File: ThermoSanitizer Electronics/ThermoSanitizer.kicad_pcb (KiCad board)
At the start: 2 copper layers, 86.4 x 59.7 mm, 17 parts, among them J1 5V_Thermo, J2 9V_In, J3 Ultrasonic, J5 Motor_Out, Q1 IRF540N, U1 L7805

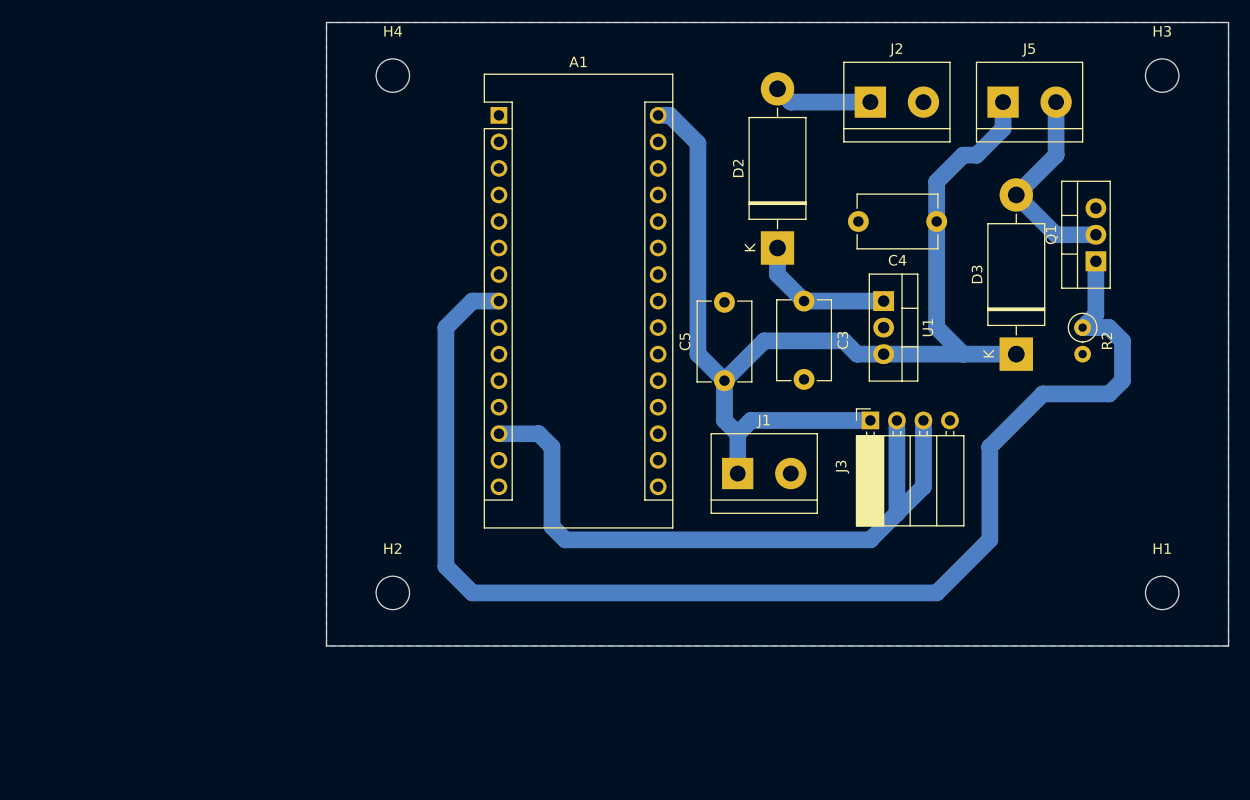
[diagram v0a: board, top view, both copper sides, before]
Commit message: Adding alot of stuff
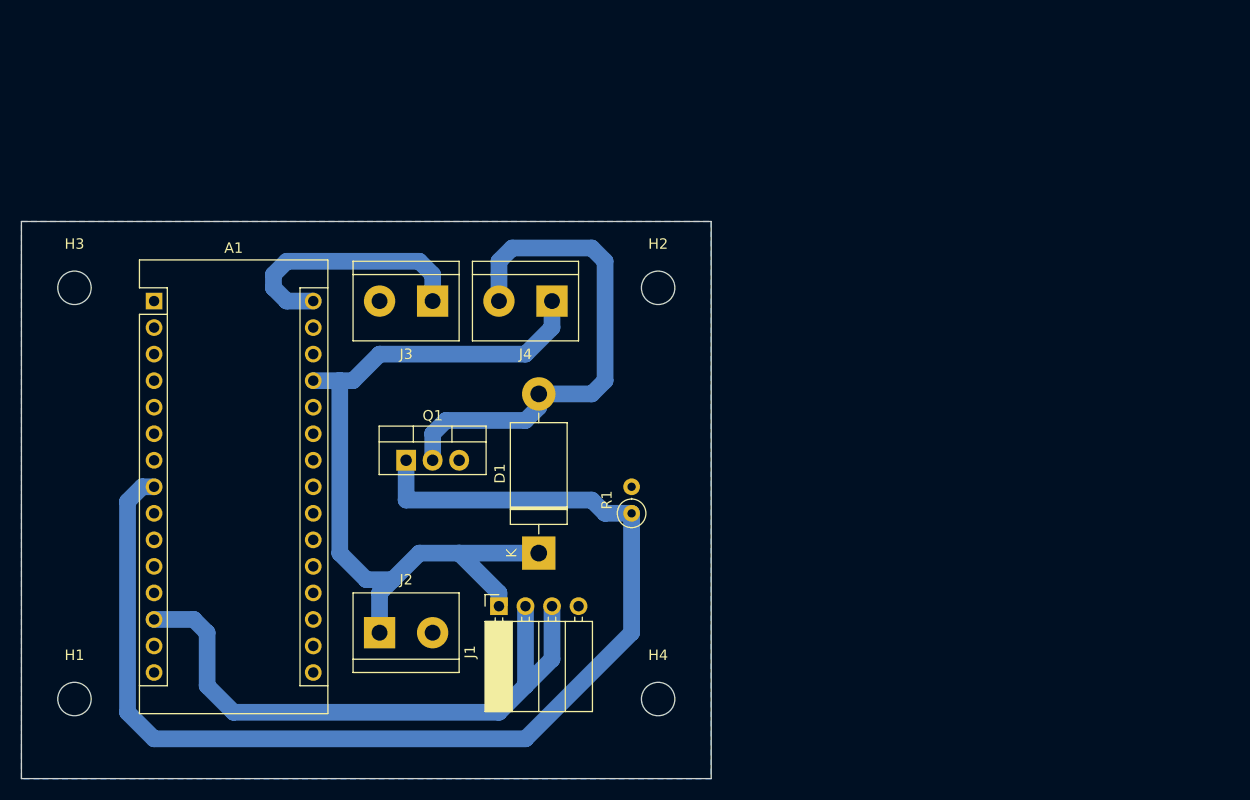
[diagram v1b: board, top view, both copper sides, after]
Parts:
- removed C3: 10uF, Capacitor_THT:C_Disc_D7.5mm_W5.0mm_P7.50mm
- removed C4: 0.1uF, Capacitor_THT:C_Disc_D7.5mm_W5.0mm_P7.50mm
- removed C5: 1uF, Capacitor_THT:C_Disc_D7.5mm_W5.0mm_P7.50mm
- removed D2, D3: 1N5400, Diode_THT:D_DO-201AD_P15.24mm_Horizontal
- removed J5: Motor_Out, TerminalBlock:TerminalBlock_bornier-2_P5.08mm
- removed R2: 1K, Resistor_THT:R_Axial_DIN0207_L6.3mm_D2.5mm_P2.54mm_Vertical
- removed U1: L7805, Package_TO_SOT_THT:TO-220-3_Vertical
- added D1: 1N5400, Diode_THT:D_DO-201AD_P15.24mm_Horizontal, F.Cu at (91.4, 97.8)
- added J4: Motor_Out, TerminalBlock:TerminalBlock_bornier-2_P5.08mm, F.Cu at (92.7, 73.7)
- added R1: 1K, Resistor_THT:R_Axial_DIN0207_L6.3mm_D2.5mm_P2.54mm_Vertical, F.Cu at (100.3, 94.0)
- H1, H2, H3, H4: value MountingHole_Pad -> MountingHole
- J1: value 5V_Thermo -> Ultrasonic; footprint TerminalBlock:TerminalBlock_bornier-2_P5.08mm -> Connector_PinSocket_2.54mm:PinSocket_1x04_P2.54mm_Horizontal
- J2: value 9V_In -> 5V_Thermo
- J3: value Ultrasonic -> 9V_In; footprint Connector_PinSocket_2.54mm:PinSocket_1x04_P2.54mm_Horizontal -> TerminalBlock:TerminalBlock_bornier-2_P5.08mm
- moved H3 106.1 mm to (47.0, 72.4)
- moved H1 104.6 mm to (47.0, 111.8)
- moved J2 69.2 mm to (76.2, 105.4)
- moved Q1 68.7 mm to (78.7, 88.9), turned to 0 degrees
- moved H4 64.9 mm to (102.9, 111.8)
- moved J3 43.4 mm to (81.3, 73.7), turned to 180 degrees
- moved H2 38.7 mm to (102.9, 72.4)
- moved A1 37.5 mm to (54.6, 73.7)
- moved J1 26.2 mm to (87.6, 102.9), turned to 90 degrees
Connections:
- net SCL renamed Net-(A1-Pad24)
- net SDA renamed Net-(A1-Pad23)
- A1 pad 27: Net-(A1-Pad27) -> +5V
- A1 pad 30: +5V -> +9V
- H1 pad 1: GND -> (no net)
- H2 pad 1: GND -> (no net)
- H3 pad 1: GND -> (no net)
- H4 pad 1: GND -> (no net)
- J1 pad 2: GND -> TRIG&ECHO
- J2 pad 1: +9V -> +5V
- J3 pad 1: +5V -> +9V
- J3 pad 2: TRIG&ECHO -> GND
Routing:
- net +5V: track 109.9 -> 77.4 mm
- net Net-(D1-Pad2): track 19.7 -> 48.4 mm
- net +9V: track 9.42 -> 24.4 mm
- net Net-(C3-Pad1): track 13.8 -> 0.00 mm
- net MOTOR: track 123.5 -> 113.9 mm
- net TRIG&ECHO: track 66.7 -> 59.6 mm
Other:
- board size 86.4 x 59.7 mm -> 66 x 53.3 mm
